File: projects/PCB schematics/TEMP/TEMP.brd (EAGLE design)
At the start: 73.7 x 76.2 mm, 58 parts, among them J1 770968-1, J2 770968-1, J3 1-770969-0, J4 770966-1

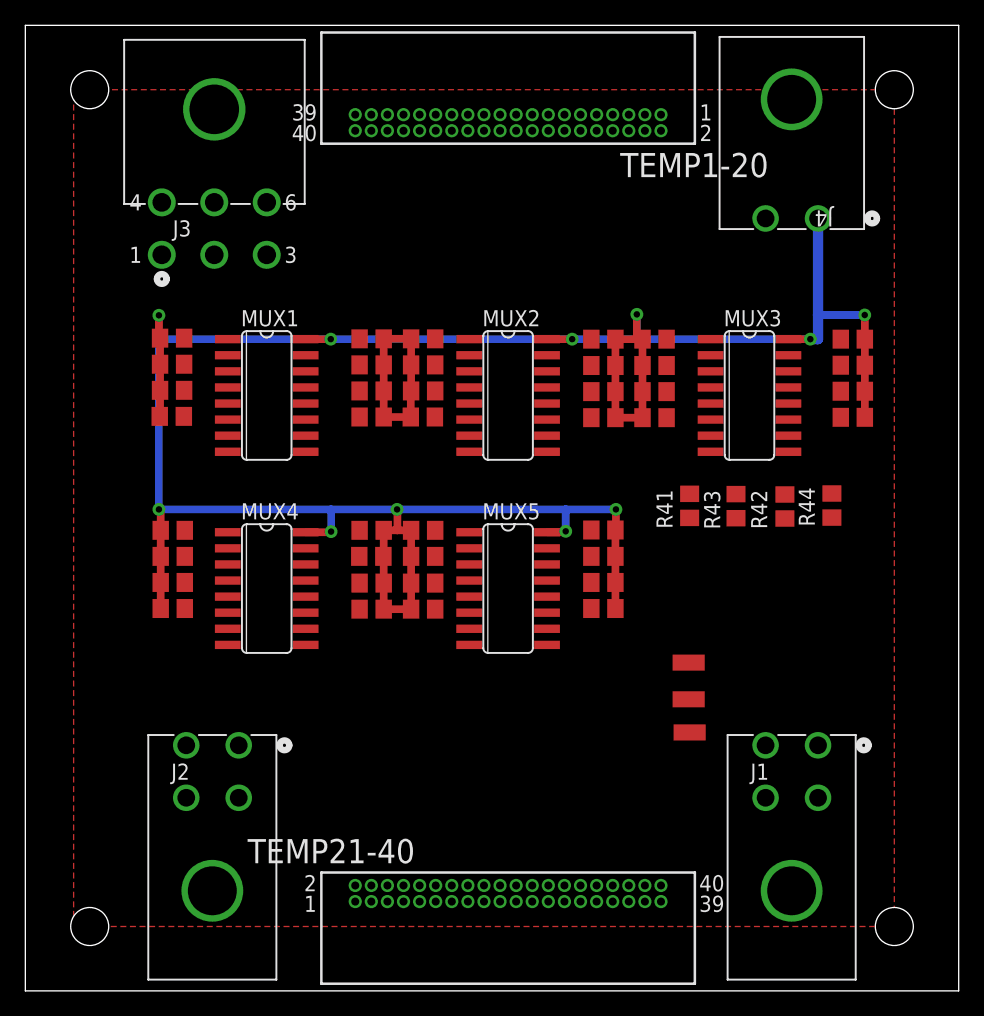
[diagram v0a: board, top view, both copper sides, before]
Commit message: TEMP - Final routing.
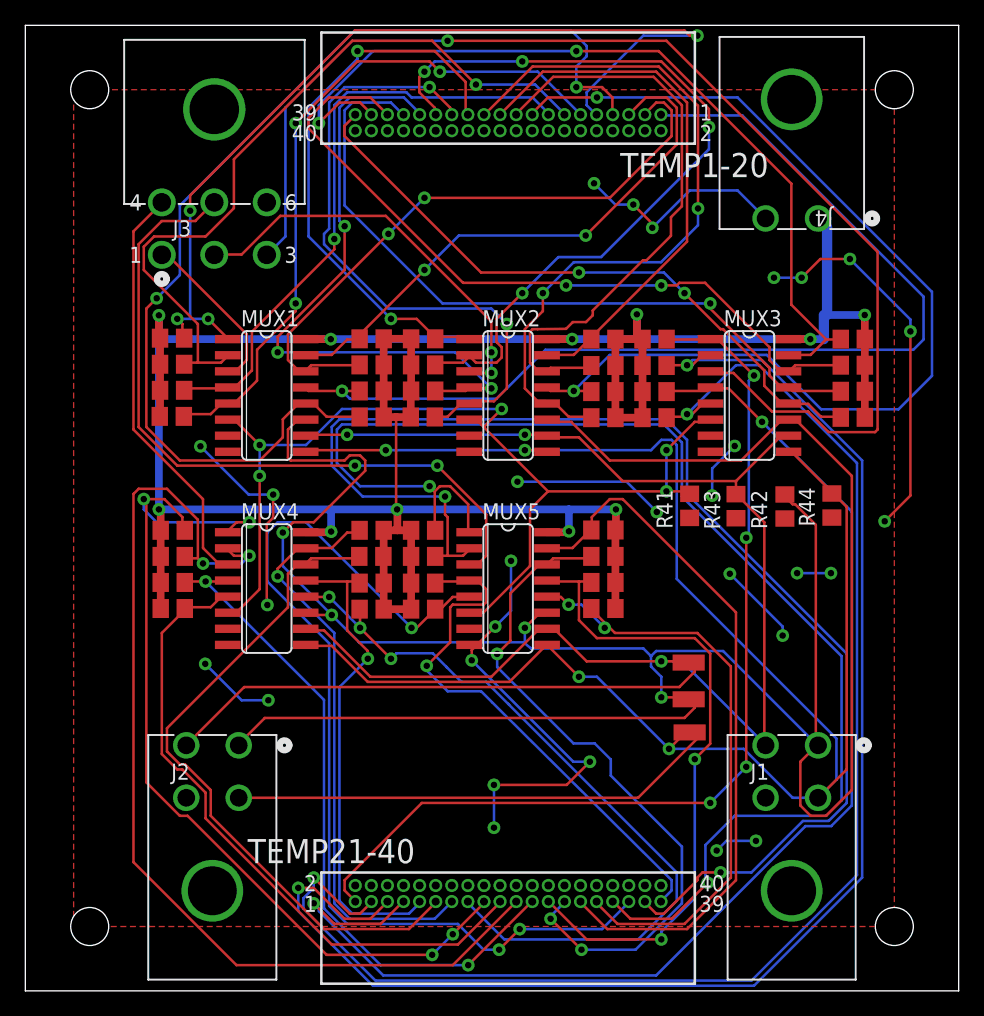
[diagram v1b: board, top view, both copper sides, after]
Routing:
- net CS_A_IN: track 0.00 -> 166.8 mm, vias 0 -> 4
- net CS_C_IN: track 0.00 -> 145.4 mm, vias 0 -> 4
- net GND: track 0.00 -> 132.7 mm, vias 0 -> 29
- net TEMP23: track 0.00 -> 115.0 mm, vias 0 -> 2
- net TEMP22: track 0.00 -> 113.3 mm, vias 0 -> 2
- net CS_B_IN: track 0.00 -> 107.9 mm, vias 0 -> 3
- net TEMP37: track 0.00 -> 105.9 mm, vias 0 -> 2
- net TEMP39: track 0.00 -> 103.7 mm, vias 0 -> 2
- net TEMP24: track 0.00 -> 101.0 mm, vias 0 -> 2
- net TEMP_OUT3: track 0.00 -> 97.3 mm, vias 0 -> 1
- net TEMP4: track 0.00 -> 86.1 mm, vias 0 -> 2
- net TEMP1: track 0.00 -> 82.6 mm, vias 0 -> 1
- net TEMP31: track 0.00 -> 81.7 mm, vias 0 -> 2
- net TEMP9: track 0.00 -> 81.1 mm, vias 0 -> 2
- net INH: track 0.00 -> 80.9 mm, vias 0 -> 5
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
